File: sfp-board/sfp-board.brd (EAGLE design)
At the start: 115.5 x 92.4 mm, 6 parts

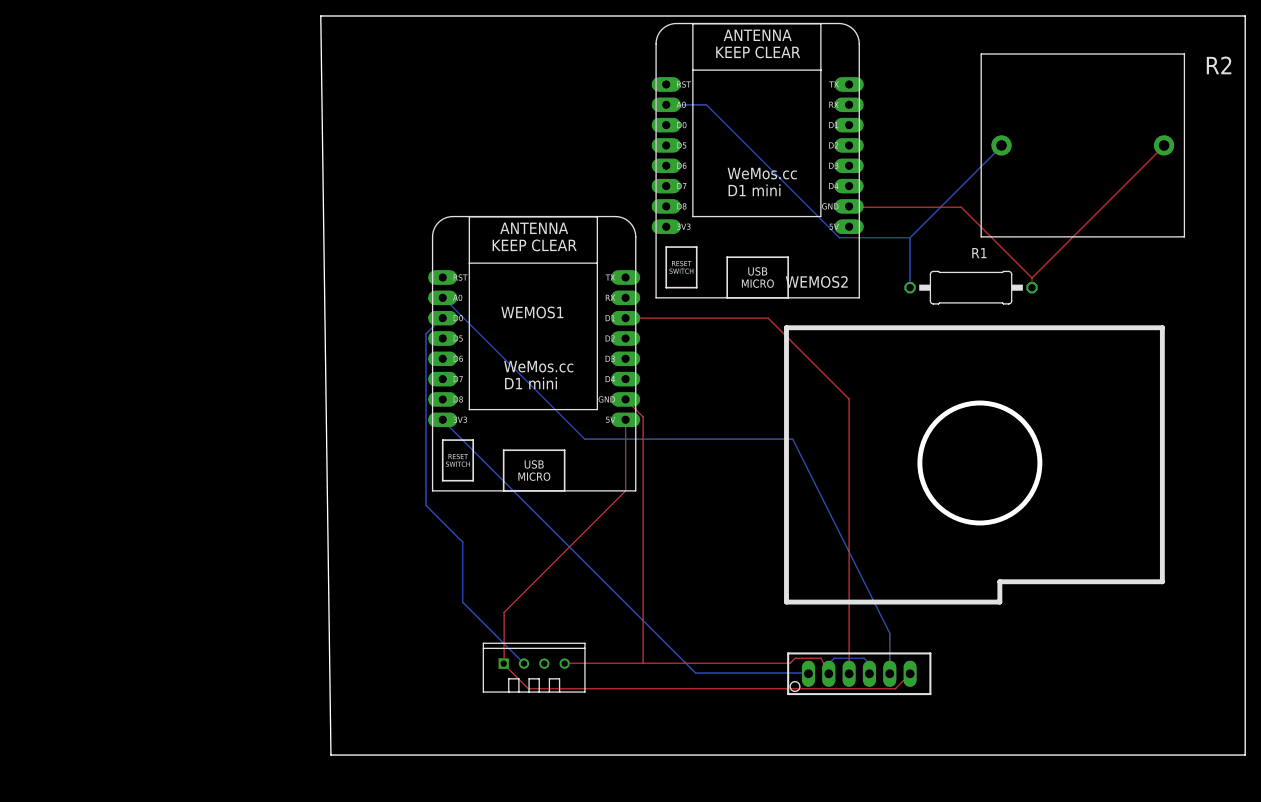
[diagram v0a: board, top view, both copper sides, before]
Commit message: Initial version sfp board
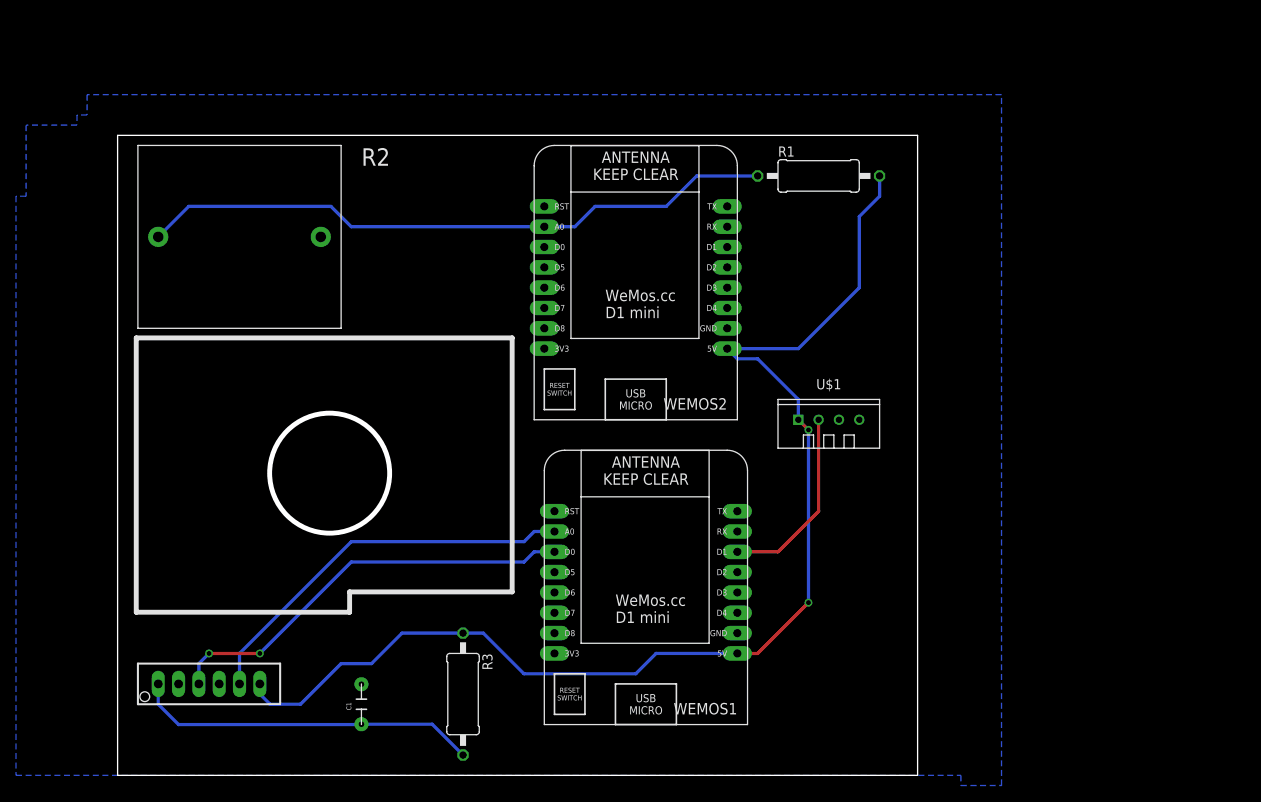
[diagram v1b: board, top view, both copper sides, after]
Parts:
- added C1: (no value), digital-toy:CAP-PTH-5MM
- added R3: 150ohm, rcl:0411/15
- moved R2 106.0 mm to (15.2, 67.3)
- moved U$2 81.3 mm to (33.0, 6.35)
- moved U$1 47.8 mm to (88.9, 44.5)
- moved WEMOS1 32.4 mm to (64.8, 25.4)
- moved R1 23.6 mm to (87.6, 74.9)
- moved WEMOS2 21.6 mm to (63.5, 63.5)
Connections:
- removed net N$1 (its old number): U$1.4, U$2.2, U$2.4, WEMOS1.GND
- removed net N$2 (its old number): R1.2, R2.2, WEMOS2.GND
- removed net N$6: U$1.1, U$2.6, WEMOS1.5V
- new net GND: C1.2, R2.2, U$1.4, U$2.2, U$2.4, WEMOS1.GND, WEMOS2.GND
- new net VCC: R1.2, R3.1, U$1.1, U$2.6, WEMOS1.5V, WEMOS2.5V
- net N$3: now also U$2.3; no longer U$1.2
- net N$4: now also C1.1, R3.2; no longer WEMOS1.3V3
- net N$7: now also U$1.2; no longer U$2.3
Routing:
- net VCC: track 0.00 -> 152.0 mm, vias 0 -> 2
- net N$6: track 89.7 -> 0.00 mm
- net N$1 (its old number): track 76.5 -> 0.00 mm
- net N$2 (its old number): track 51.2 -> 0.00 mm
- net N$7: track 66.5 -> 23.7 mm
- net N$1: track 83.3 -> 49.5 mm
- net N$2: track 59.9 -> 80.2 mm
- net N$4: track 58.9 -> 43.3 mm
- net N$3: track 49.2 -> 52.8 mm, vias 0 -> 2
- added copper zone on layer 16, net GND
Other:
- board size 115.5 x 92.4 mm -> 100 x 80 mm
